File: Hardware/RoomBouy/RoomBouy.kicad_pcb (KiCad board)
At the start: 2 copper layers, 65 x 56.5 mm, 1 part, among them J2 Raspberry_Pi_2_3

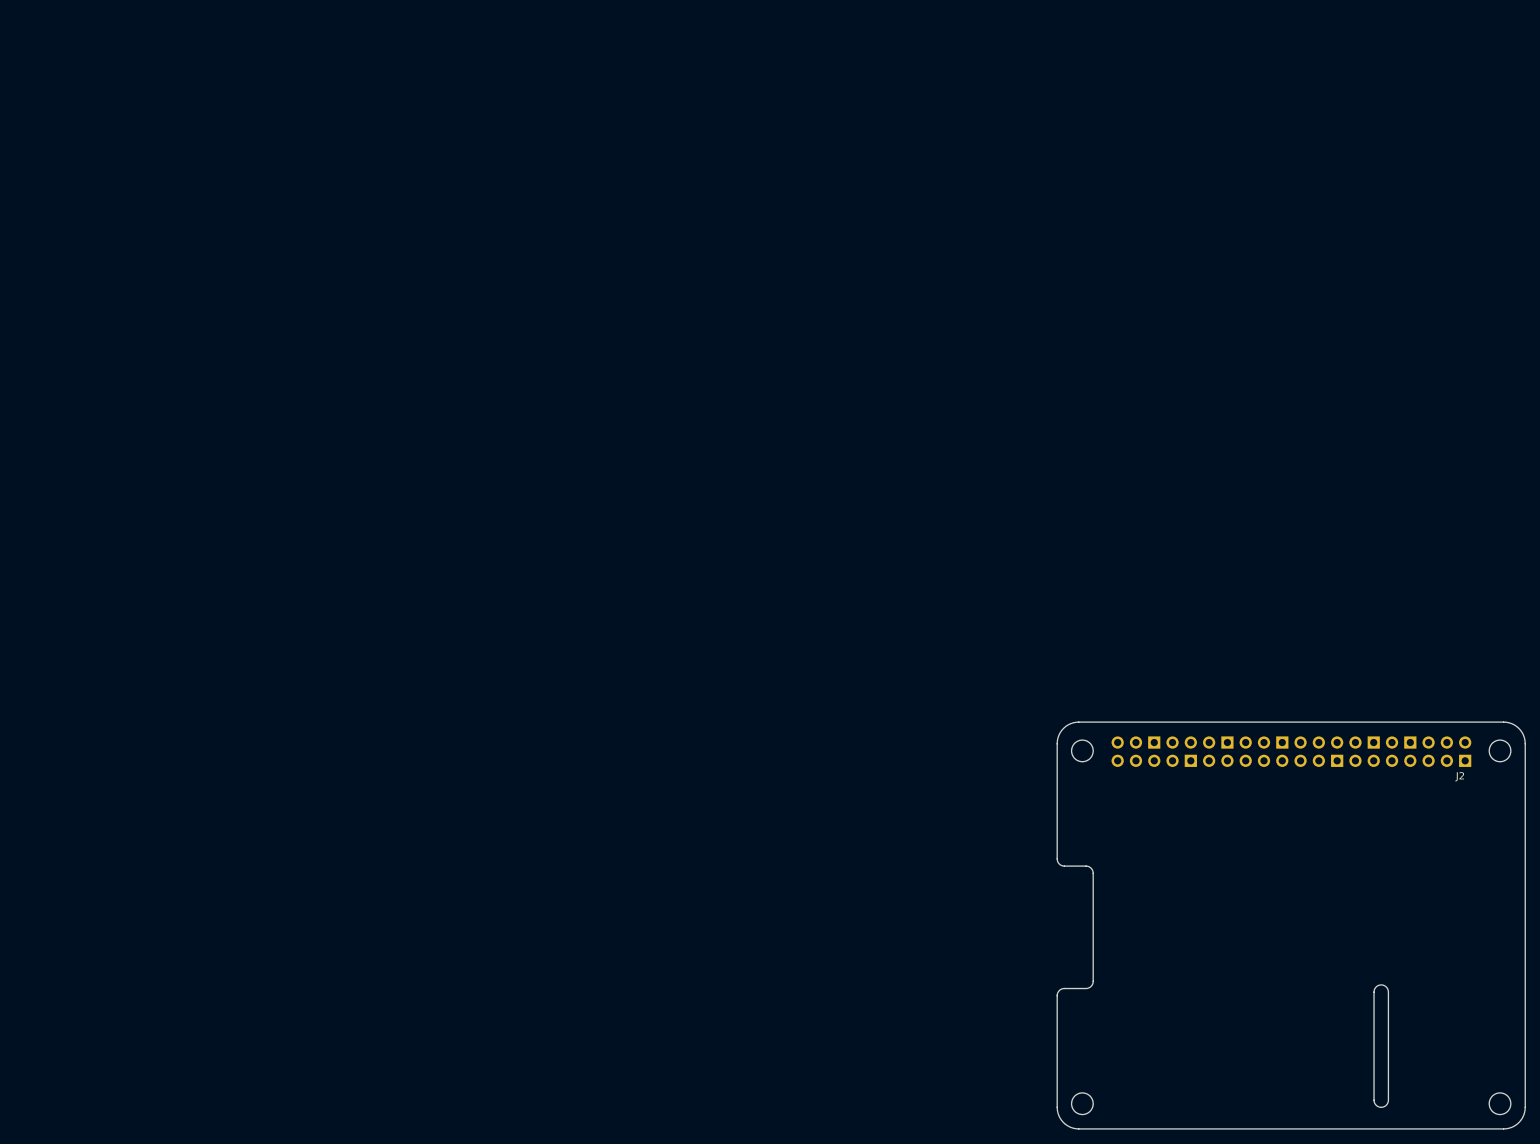
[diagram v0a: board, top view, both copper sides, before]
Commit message: Clean sheet
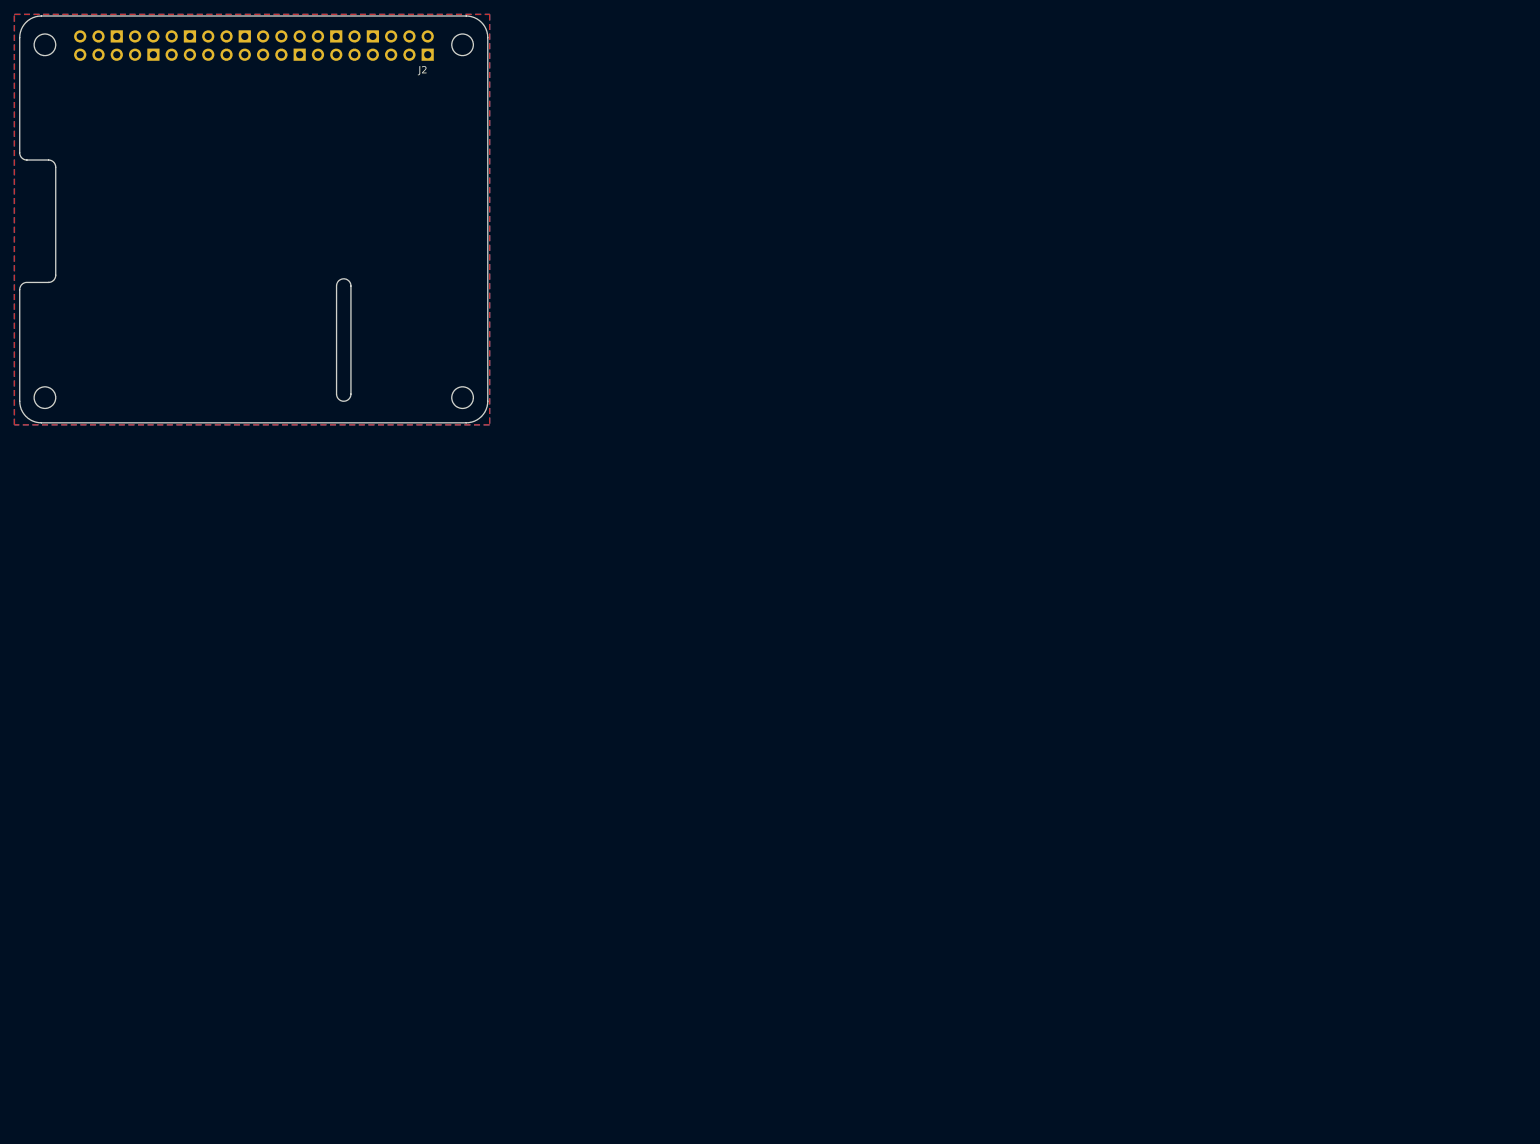
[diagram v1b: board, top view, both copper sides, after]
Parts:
- moved J2 174.3 mm to (0.16, -24.8)
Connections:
- net Net-(J2-GND-Pad14) renamed GND
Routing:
- added copper zone on B.Cu, net GND
- added copper zone on F.Cu, net GND
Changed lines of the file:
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@@
 	(net 1 "unconnected-(J2-GPIO26-Pad37)")
 	(net 2 "Net-(J2-5V-Pad2)")
-	(net 3 "Net-(J2-GND-Pad14)")
+	(net 3 "GND")
 	(net 4 "unconnected-(J2-~{CE1}{slash}GPIO7-Pad26)")
 	(net 5 "unconnected-(J2-GPIO23-Pad16)")
@@
 	(footprint "RPI_Hat:RPI_Hat_B+"
 		(layer "F.Cu")
-		(at 144.24 73.222)
+		(at 0.16 -24.838)
 		(property "Reference" "J2"
 			(at 23.5 3.5 0)
@@
 			(layer "Dwgs.User")
 			(pts
-				(xy 115.24 126.722) (xy 111.74 126.722)
+				(xy -28.84 28.662) (xy -32.34 28.662)
 			)
 			(height -2.5)
 			(gr_text "3.5000 mm"
-				(at 113.49 127.572 0)
+				(at -30.59 29.512 0)
 				(layer "Dwgs.User")
 				(effects
@@
 			(layer "Dwgs.User")
 			(pts
-				(xy 158.74 122.722) (xy 158.74 105.722)
+				(xy 14.66 24.662) (xy 14.66 7.662)
 			)
 			(height 3)
 			(gr_text "17.0000 mm"
-				(at 160.09 114.222 90)
+				(at 16.01 16.162 90)
 				(layer "Dwgs.User")
 				(effects
@@
 			(layer "Dwgs.User")
 			(pts
-				(xy 154.74 125.722) (xy 154.74 114.222)
+				(xy 10.66 27.662) (xy 10.66 16.162)
 			)
 			(height -2.499999)
 			(gr_text "11.5000 mm"
-				(at 150.590001 119.972 90)
+				(at 6.510001 21.912 90)
 				(layer "Dwgs.User")
 				(effects
@@
 			(layer "Dwgs.User")
 			(pts
-				(xy 176.74 68.222) (xy 111.74 68.222)
+				(xy 32.66 -29.838) (xy -32.34 -29.838)
 			)
 			(height 7)
 			(gr_text "65.0000 mm"
-				(at 144.24 59.572 0)
+				(at 0.16 -38.488 0)
 				(layer "Dwgs.User")
 				(effects
@@
 			(layer "Dwgs.User")
 			(pts
-				(xy 110.74 125.722) (xy 110.74 106.222)
+				(xy -33.34 27.662) (xy -33.34 8.162)
 			)
 			(height -3)
 			(gr_text "19.5000 mm"
-				(at 106.09 115.972 90)
+				(at -37.99 17.912 90)
 				(layer "Dwgs.User")
 				(effects
@@
 			(layer "Dwgs.User")
 			(pts
-				(xy 177.74 125.722) (xy 177.74 69.722)
+				(xy 33.66 27.662) (xy 33.66 -28.338)
 			)
 			(height 8)
 			(gr_text "56.0000 mm"
-				(at 184.09 97.722 90)
+				(at 40.01 -0.338 90)
 				(layer "Dwgs.User")
 				(effects
@@
 			(layer "Dwgs.User")
 			(pts
-				(xy 157.74 104.722) (xy 155.74 104.722)
+				(xy 13.66 6.662) (xy 11.66 6.662)
 			)
 			(height 2.499999)
 			(gr_text "2.0000 mm"
-				(at 156.74 100.572001 0)
+				(at 12.66 2.512001 0)
 				(layer "Dwgs.User")
 				(effects
@@
 			(layer "Dwgs.User")
 			(pts
-				(xy 173.24 68.222) (xy 115.24 68.222)
+				(xy 29.16 -29.838) (xy -28.84 -29.838)
 			)
 			(height 2.5)
 			(gr_text "58.0000 mm"
-				(at 144.24 64.072 0)
+				(at 0.16 -33.988 0)
 				(layer "Dwgs.User")
 				(effects
@@
 			(layer "Dwgs.User")
 			(pts
-				(xy 177.74 122.222) (xy 177.74 73.222)
+				(xy 33.66 24.162) (xy 33.66 -24.838)
 			)
 			(height 2.999999)
 			(gr_text "49.0000 mm"
-				(at 179.089999 97.722 90)
+				(at 35.009999 -0.338 90)
 				(layer "Dwgs.User")
 				(effects
@@
 			(layer "Dwgs.User")
 			(pts
-				(xy 177.74 125.722) (xy 177.74 69.222)
+				(xy 33.66 27.662) (xy 33.66 -28.838)
 			)
 			(height 12)
 			(gr_text "56.5000 mm"
-				(at 188.09 97.472 90)
+				(at 44.01 -0.588 90)
 				(layer "Dwgs.User")
 				(effects
@@
 			(layer "Dwgs.User")
 			(pts
-				(xy 116.74 89.222) (xy 111.74 89.222)
+				(xy -27.34 -8.838) (xy -32.34 -8.838)
 			)
 			(height 2)
 			(gr_text "5.0000 mm"
-				(at 114.24 85.572 0)
+				(at -29.84 -12.488 0)
 				(layer "Dwgs.User")
 				(effects
@@
 			(layer "Dwgs.User")
 			(pts
-				(xy 118.74 125.722) (xy 118.74 122.222)
+				(xy -25.34 27.662) (xy -25.34 24.162)
 			)
 			(height 3)
 			(gr_text "3.5000 mm"
-				(at 120.09 123.972 90)
+				(at -23.99 25.912 90)
 				(layer "Dwgs.User")
 				(effects
@@
 			(layer "Dwgs.User")
 			(pts
-				(xy 144.24 75.222001) (xy 115.24 75.222001)
+				(xy 0.16 -22.837999) (xy -28.84 -22.837999)
 			)
 			(height -2.499999)
 			(gr_text "29.0000 mm"
-				(at 129.74 79.722001 0)
+				(at -14.34 -18.337999 0)
 				(layer "Dwgs.User")
 				(effects
@@
 			(layer "Dwgs.User")
 			(pts
-				(xy 117.74 106.222) (xy 117.74 89.222)
+				(xy -26.34 8.162) (xy -26.34 -8.838)
 			)
 			(height 2)
 			(gr_text "17.0000 mm"
-				(at 118.09 97.722 90)
+				(at -25.99 -0.338 90)
 				(layer "Dwgs.User")
 				(effects
@@
 			(layers "*.Cu" "*.Mask")
 			(remove_unused_layers no)
-			(net 3 "Net-(J2-GND-Pad14)")
+			(net 3 "GND")
 			(pinfunction "GND")
 			(pintype "power_in")
@@
 			(layers "*.Cu" "*.Mask")
 			(remove_unused_layers no)
-			(net 3 "Net-(J2-GND-Pad14)")
+			(net 3 "GND")
 			(pinfunction "GND")
 			(pintype "passive")
@@
 			(layers "*.Cu" "*.Mask")
 			(remove_unused_layers no)
-			(net 3 "Net-(J2-GND-Pad14)")
+			(net 3 "GND")
 			(pinfunction "GND")
 			(pintype "passive")
@@
 			(layers "*.Cu" "*.Mask")
 			(remove_unused_layers no)
-			(net 3 "Net-(J2-GND-Pad14)")
+			(net 3 "GND")
 			(pinfunction "GND")
 			(pintype "passive")
@@
 			(layers "*.Cu" "*.Mask")
 			(remove_unused_layers no)
-			(net 3 "Net-(J2-GND-Pad14)")
+			(net 3 "GND")
 			(pinfunction "GND")
 			(pintype "passive")
@@
 			(layers "*.Cu" "*.Mask")
 			(remove_unused_layers no)
-			(net 3 "Net-(J2-GND-Pad14)")
+			(net 3 "GND")
 			(pinfunction "GND")
 			(pintype "passive")
@@
 			(layers "*.Cu" "*.Mask")
 			(remove_unused_layers no)
-			(net 3 "Net-(J2-GND-Pad14)")
+			(net 3 "GND")
 			(pinfunction "GND")
 			(pintype "passive")
@@
 			(layers "*.Cu" "*.Mask")
 			(remove_unused_layers no)
-			(net 3 "Net-(J2-GND-Pad14)")
+			(net 3 "GND")
 			(pinfunction "GND")
 			(pintype "passive")
@@
 		)
 	)
+	(zone
+		(net 3)
+		(net_name "GND")
+		(layers "F&B.Cu")
+		(hatch edge 0.5)
+		(connect_pads
+			(clearance 0.5)
+		)
+		(min_thickness 0.25)
+		(filled_areas_thickness no)
+		(fill yes
+			(thermal_gap 0.5)
+			(thermal_bridge_width 0.5)
+		)
+		(polygon
+			(pts
+				(xy 32.92 -29.06) (xy 32.92 27.94) (xy -33.08 27.94) (xy -33.08 -29.06)
+			)
+		)
+	)
